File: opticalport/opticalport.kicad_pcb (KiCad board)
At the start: 2 copper layers, 30.5 x 16.5 mm, 15 parts, among them J1 Conn_02x03_Odd_Even, Q1 APTD3216P3C-P22, Q2 BC817, Q3 APTD3216P3C-P22, Q4 BC817

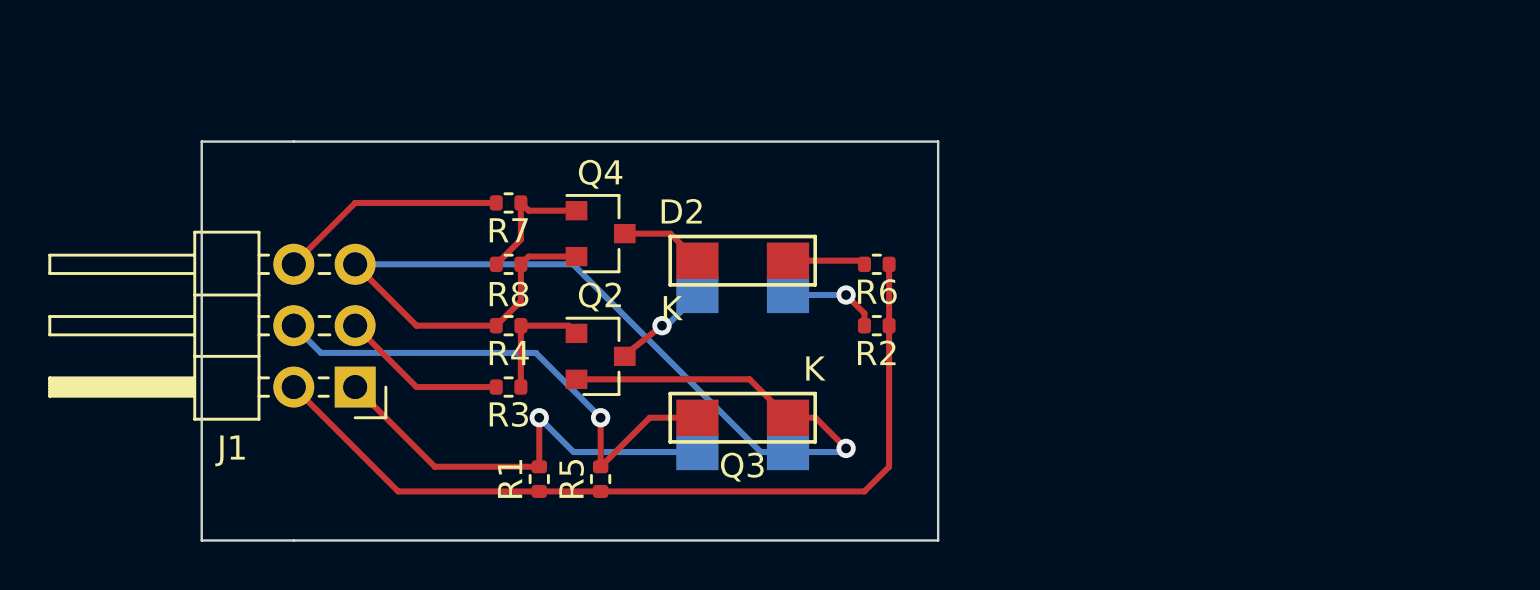
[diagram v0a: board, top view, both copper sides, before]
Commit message: Update schematic and layout
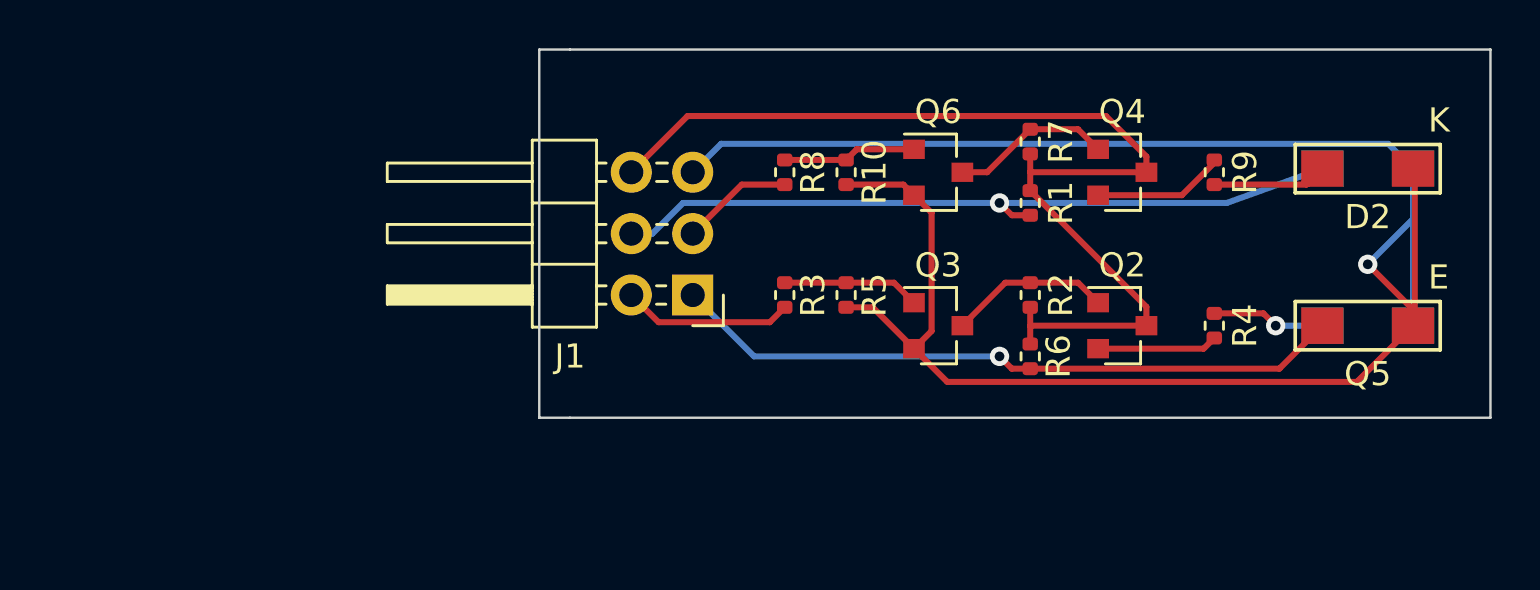
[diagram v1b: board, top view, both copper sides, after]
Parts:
- added Q5: APTD3216P3C-P22, opticalport:LED_Kingbright_APTD3216, F.Cu at (166.4, 87.6)
- added Q6: BC817, Package_TO_SOT_SMD:SOT-23, F.Cu at (148.6, 81.3)
- added R10: 1.5k, Resistor_SMD:R_0402_1005Metric, F.Cu at (144.8, 81.3)
- added R9: 91, Resistor_SMD:R_0402_1005Metric, F.Cu at (160.0, 81.3)
- Q3: value APTD3216P3C-P22 -> BC817; footprint opticalport:LED_Kingbright_APTD3216 -> Package_TO_SOT_SMD:SOT-23
- R2: value 100 -> 330
- R3: value 4.7k -> 5.1k
- R4: value 1.5k -> 91
- R5: value 2.2K -> 1.5k
- R6: value 100 -> 2.2K
- R7: value 4.7K -> 330
- R8: value 1.5K -> 5.1k
- moved R4 29.2 mm to (160.0, 87.6), turned to 90 degrees
- moved Q1 28.4 mm to (166.4, 81.1)
- moved D2 26.1 mm to (166.4, 81.1), turned to 180 degrees
- moved D1 25.9 mm to (166.4, 87.6), turned to 180 degrees
- moved R1 23.3 mm to (152.4, 82.5), turned to 270 degrees
- moved Q4 21.7 mm to (156.2, 81.3)
- moved R7 21.7 mm to (152.4, 80.0), turned to 90 degrees
- moved Q2 21.6 mm to (156.2, 87.6)
- moved J1 14.5 mm to (138.4, 86.4)
- moved R5 12.7 mm to (144.8, 86.4), turned to 270 degrees
- moved R3 12.0 mm to (142.2, 86.4), turned to 270 degrees
- moved R8 12.0 mm to (142.2, 81.3), turned to 270 degrees
- moved Q3 8.94 mm to (148.6, 87.6), turned to 0 degrees
- moved R6 7.41 mm to (152.4, 88.9), turned to 270 degrees
- moved R2 6.48 mm to (152.4, 86.4), turned to 90 degrees
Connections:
- D1 pad 1: Net-(D1-Pad1) -> GND
- D2 pad 1: Net-(D2-Pad1) -> GND
- J1 pad 2: +3V3 -> TX1
- J1 pad 6: TX1 -> +3V3
- Q1 pad 2: RX2 -> RX1
- Q2 pad 2: GND -> Net-(Q2-Pad2)
- Q2 pad 3: Net-(D1-Pad1) -> +3V3
- Q3 pad 1: GND -> Net-(Q3-Pad1)
- Q3 pad 2: RX1 -> GND
- Q4 pad 2: GND -> Net-(Q4-Pad2)
- Q4 pad 3: Net-(D2-Pad1) -> +3V3
- R1 pad 2: RX2 -> RX1
- R2 pad 2: Net-(D1-Pad2) -> Net-(Q2-Pad1)
- R3 pad 1: Net-(Q2-Pad1) -> Net-(Q3-Pad1)
- R3 pad 2: TX2 -> TX1
- R4 pad 1: Net-(Q2-Pad1) -> Net-(Q2-Pad2)
- R4 pad 2: GND -> Net-(D1-Pad2)
- R5 pad 1: +3V3 -> Net-(Q3-Pad1)
- R5 pad 2: RX1 -> GND
- R6 pad 2: Net-(D2-Pad2) -> RX2
- R7 pad 1: Net-(Q4-Pad1) -> +3V3
- R7 pad 2: TX1 -> Net-(Q4-Pad1)
- R8 pad 1: Net-(Q4-Pad1) -> Net-(Q6-Pad1)
- R8 pad 2: GND -> TX2
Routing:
- net GND: track 48.2 -> 85.5 mm
- net RX1: track 21.2 -> 31.4 mm
- net RX2: track 18.2 -> 28.1 mm
- net +3V3: track 35.2 -> 44.1 mm
- net Net-(Q3-Pad1): track 0.00 -> 5.69 mm
- net Net-(Q6-Pad1): track 0.00 -> 5.53 mm
- net Net-(Q4-Pad2): track 0.00 -> 5.48 mm
- net Net-(Q2-Pad2): track 0.00 -> 4.99 mm
- net Net-(D1-Pad1): track 3.99 -> 0.00 mm, vias 1 -> 0
- net Net-(D2-Pad1): track 3.47 -> 0.00 mm
- net TX1: track 9.43 -> 7.07 mm
- net TX2: track 6.89 -> 4.65 mm
- net Net-(Q2-Pad1): track 4.97 -> 6.70 mm
- net Net-(D2-Pad2): track 3.23 -> 4.75 mm
- net Net-(Q4-Pad1): track 5.40 -> 6.70 mm
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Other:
- board size 30.5 x 16.5 mm -> 39.4 x 15.2 mm
- board text added: "Optopod v1.0 E. Beroset"
